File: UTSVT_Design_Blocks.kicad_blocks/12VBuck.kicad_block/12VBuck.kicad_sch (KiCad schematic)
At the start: 9 parts, among them U3 LMR51635XDDCR

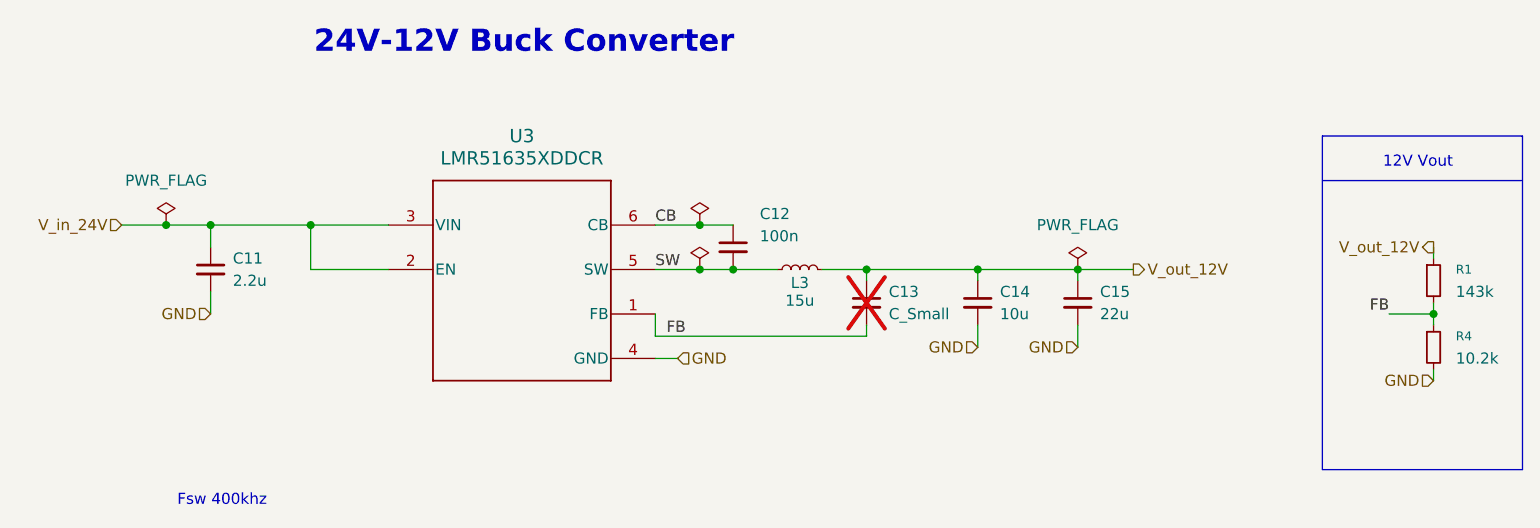
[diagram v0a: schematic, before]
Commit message: made changes
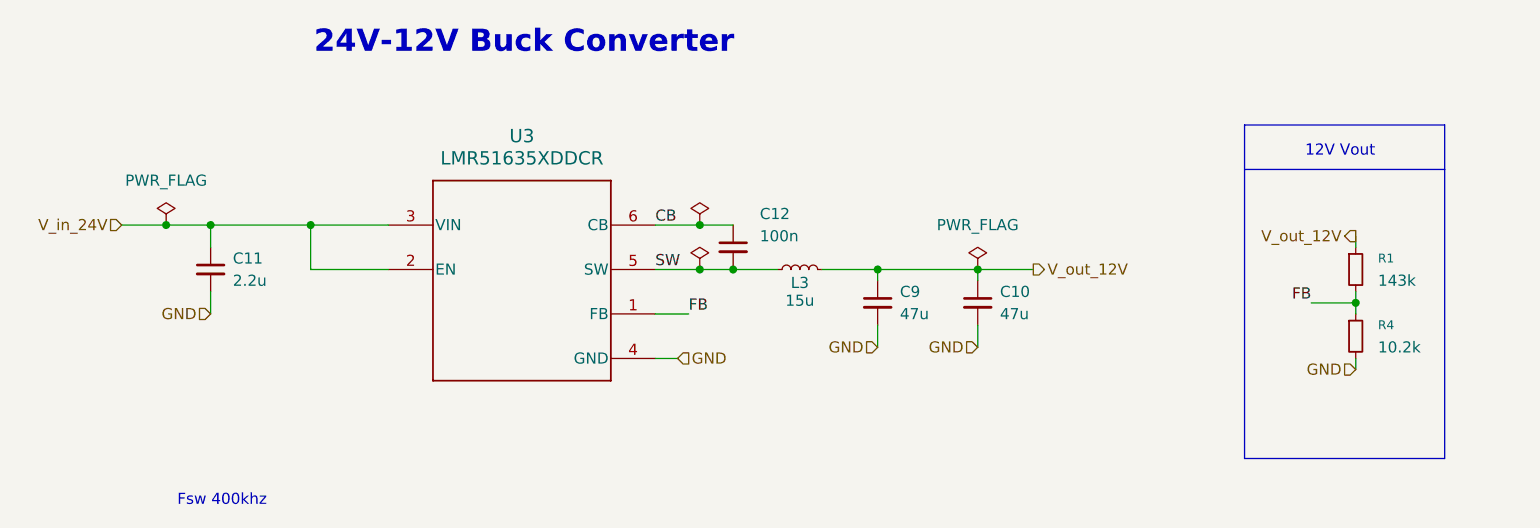
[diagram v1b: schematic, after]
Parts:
- removed C13: C_Small, Capacitor_SMD:C_0603_1608Metric_Pad1.08x0.95mm_HandSolder, symbol Device:C_Small
- removed C14: 10u, Capacitor_SMD:C_0805_2012Metric_Pad1.18x1.45mm_HandSolder, symbol Device:C_Small
- removed C15: 22u, Capacitor_SMD:C_0805_2012Metric_Pad1.18x1.45mm_HandSolder, symbol Device:C_Small
- added C10, C9: 47u, Capacitor_SMD:C_1210_3225Metric_Pad1.33x2.70mm_HandSolder, symbol Device:C_Small
- C11: footprint Capacitor_SMD:C_0603_1608Metric_Pad1.08x0.95mm_HandSolder -> Capacitor_SMD:C_0805_2012Metric_Pad1.18x1.45mm_HandSolder; LCSC P/N C1607 -> C1771; P/N 581-0603YC225MAT2A -> 963-T21GCB7225MTPA1J
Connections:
- net GND: now also C10.2, C9.2
- net V_out_12V: now also C10.1, C9.1
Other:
- moved on the sheet: R1, R4

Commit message: review addressed
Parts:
- C10, C9: P/N 963-MLAST32MAB5476MP -> GRM32ER61C476KE15L
- C11: P/N 963-T21GCB7225MTPA1J -> CL21F225ZAFNNNE
- L3: footprint Inductor_SMD:L_Cenker_CKCS4030 -> Inductor_SMD:L_TDK_VLP8040; LCSC P/N C354591 -> C2849555; P/N 504-HPAL1V1265-150-R -> PNLS8040-150M 15UH
- R1: P/N 603-RT0603DRE07143KL -> 0603WAF1433T5E
- R4: P/N 603-RT0603DRE0710K2L -> 0603WAF1022T5E
- U3: footprint breh:DDC0006A-MFG -> utsvt_ics:DDC0006A-MFG; P/N 595-LMR51635XDDCR -> LMR51635XDDCR
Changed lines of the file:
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@@
 			)
 		)
-		(property "P/N" "963-MLAST32MAB5476MP"
+		(property "P/N" "GRM32ER61C476KE15L"
 			(at 170.18 90.17 0)
 			(effects
@@
 			)
 		)
-		(property "P/N" "963-T21GCB7225MTPA1J"
+		(property "P/N" "CL21F225ZAFNNNE"
 			(at 93.98 86.36 0)
 			(effects
@@
 			)
 		)
-		(property "Footprint" "Inductor_SMD:L_Cenker_CKCS4030"
+		(property "Footprint" "Inductor_SMD:L_TDK_VLP8040"
 			(at 161.29 86.36 0)
 			(effects
@@
 			)
 		)
-		(property "LCSC P/N" "C354591"
+		(property "LCSC P/N" "C2849555"
 			(at 161.29 86.36 90)
 			(effects
@@
 			)
 		)
-		(property "P/N" "504-HPAL1V1265-150-R"
+		(property "P/N" "PNLS8040-150M 15UH"
 			(at 161.29 86.36 90)
 			(effects
@@
 			)
 		)
-		(property "Footprint" "breh:DDC0006A-MFG"
+		(property "Footprint" "utsvt_ics:DDC0006A-MFG"
 			(at 114.3 81.28 0)
 			(effects
@@
 			)
 		)
-		(property "P/N" "595-LMR51635XDDCR"
+		(property "P/N" "LMR51635XDDCR"
 			(at 114.3 81.28 0)
 			(effects
@@
 			)
 		)
-		(property "P/N" "963-MLAST32MAB5476MP"
+		(property "P/N" "GRM32ER61C476KE15L"
 			(at 181.61 90.17 0)
 			(effects
@@
 			)
 		)
-		(property "P/N" "603-RT0603DRE07143KL"
+		(property "P/N" "0603WAF1433T5E"
 			(at 224.79 86.36 0)
 			(effects
@@
 			)
 		)
-		(property "P/N" "603-RT0603DRE0710K2L"
+		(property "P/N" "0603WAF1022T5E"
 			(at 224.79 93.98 0)
 			(effects
